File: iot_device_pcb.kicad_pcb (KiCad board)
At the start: 2 copper layers, 71 parts, among them J1 B2B-PH-K-S_LF__SN_, J2 USB_C_Receptacle_USB2.0_16P, J3 Screw_Terminal_01x03, J4 Conn_01x04_Pin, J5 Conn_01x04_Pin, J6 Conn_01x07_Pin, K1 RAYEX-L90, Q1 BC817, Q2 BC817, Q3 BC817, U1 AMS1117-3.3, U2 MCP73871, U4 ESP32-S3-WROOM-1, U5 BME280, U6 MPU-6050

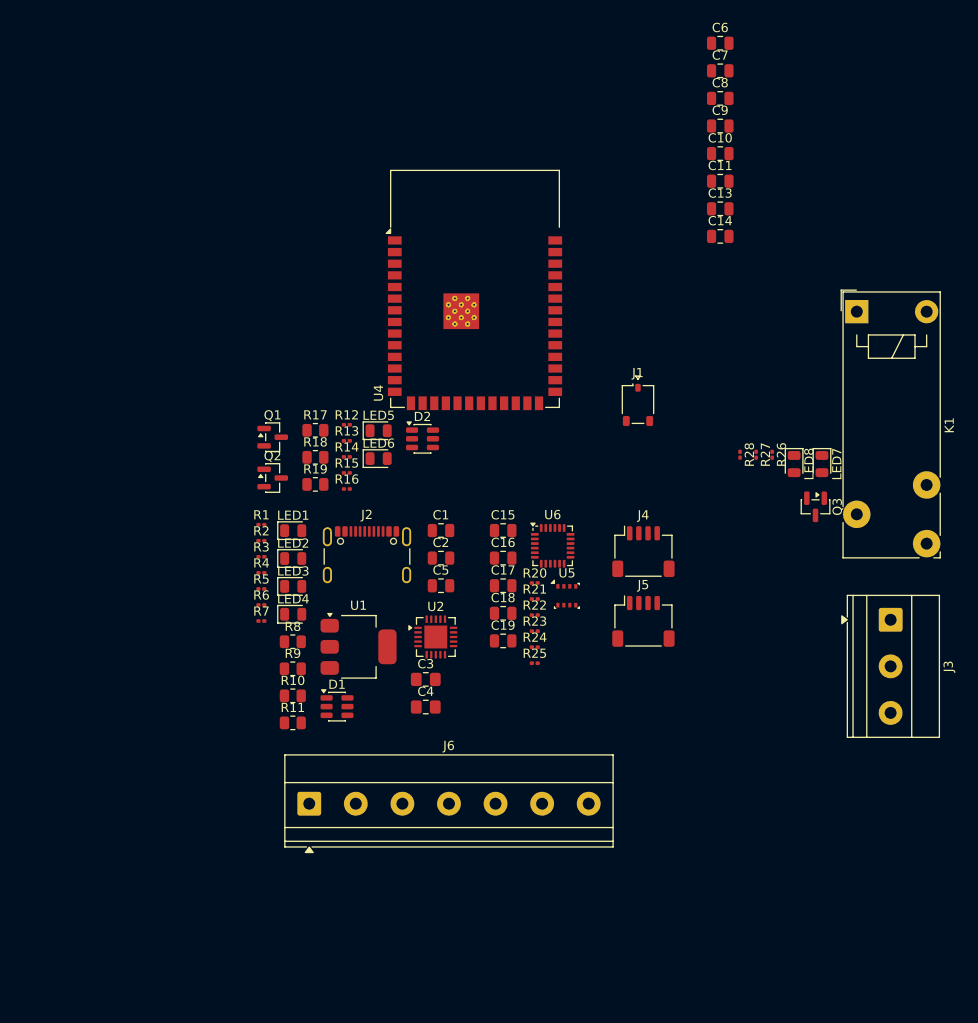
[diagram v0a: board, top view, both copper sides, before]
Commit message: Implement feature X to enhance user experience and fix bug Y in module Z
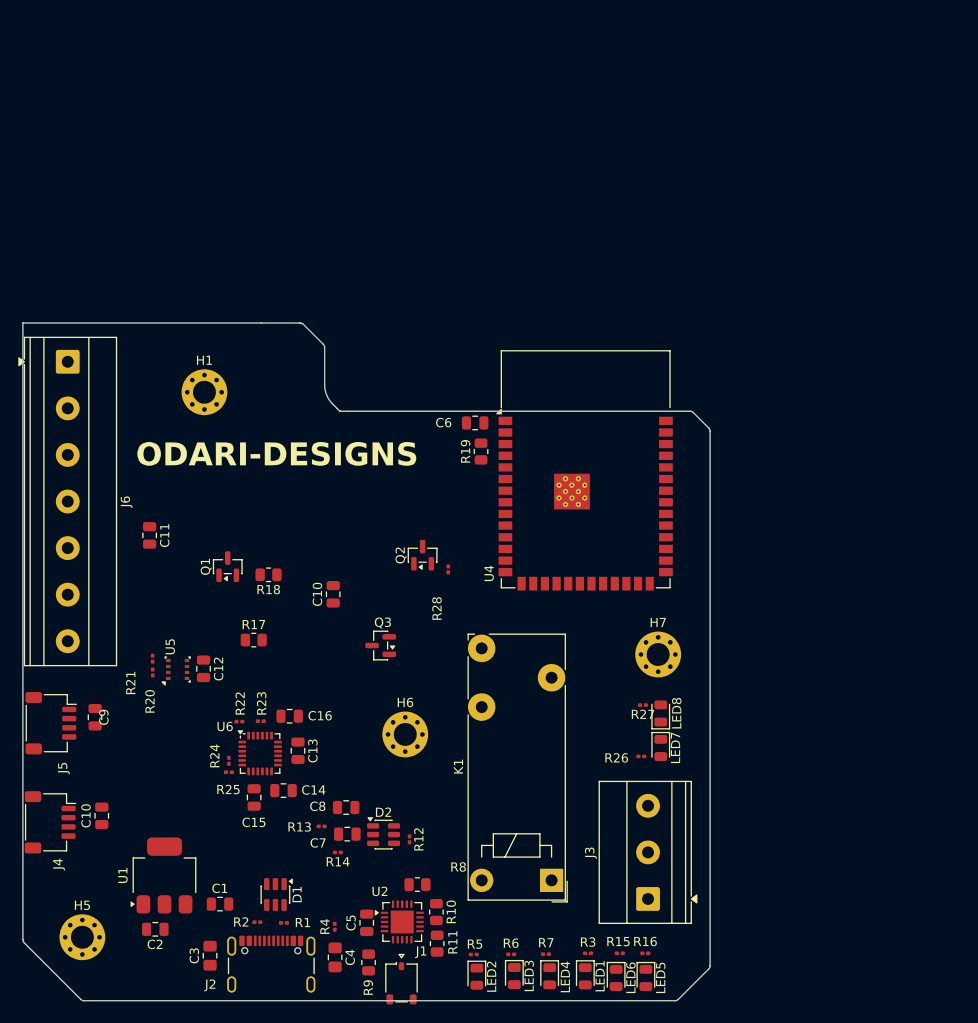
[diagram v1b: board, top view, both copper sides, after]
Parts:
- removed the C7 at (162.4, 55.2)
- added H1: MountingHole, MountingHole:MountingHole_2.5mm_Pad_Via, F.Cu at (106.1, 90.3)
- added H5: MountingHole, MountingHole:MountingHole_2.5mm_Pad_Via, F.Cu at (92.8, 149.7)
- added H6: MountingHole, MountingHole:MountingHole_2.5mm_Pad_Via, F.Cu at (128.0, 127.6)
- added H7: MountingHole, MountingHole:MountingHole_2.5mm_Pad_Via, F.Cu at (155.6, 118.9)
- moved C10 98.8 mm to (94.9, 136.5), turned to 90 degrees
- moved C9 93.9 mm to (94.2, 125.8), turned to 90 degrees
- moved C7 90.0 mm to (121.7, 138.5)
- moved C8 79.6 mm to (121.6, 135.6), turned to 180 degrees
- moved J4 71.1 mm to (89.3, 137.2), turned to -90 degrees
- moved K1 70.4 mm to (144.0, 143.5), turned to 90 degrees
- moved C11 70.3 mm to (100.1, 105.9), turned to -90 degrees
- moved J1 68.2 mm to (127.6, 154.8)
- moved LED5 66.4 mm to (154.2, 154.2), turned to -90 degrees
- moved J5 65.6 mm to (89.3, 126.4), turned to -90 degrees
- moved LED6 62.3 mm to (151.0, 154.2), turned to -90 degrees
- moved R15 60.3 mm to (151.4, 151.5), turned to 180 degrees
- moved R16 60.2 mm to (154.2, 151.5), turned to 180 degrees
- moved C10 59.6 mm to (120.1, 112.3), turned to 90 degrees
- moved LED1 58.1 mm to (147.6, 154.0), turned to -90 degrees
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- renumbered C13 to C10, C14 to C11, C15 to C12, C16 to C13, C17 to C14, C18 to C15, C19 to C16, C8 to C7, C11 to C8
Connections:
- U4 pad 12: unconnected-(U4-IO8-Pad12) -> /Microcontroller-ESP32-S3-WROOM-1/SDA
- U4 pad 15: unconnected-(U4-IO3-Pad15) -> /Microcontroller-ESP32-S3-WROOM-1/GPIO1
- U4 pad 17: unconnected-(U4-IO9-Pad17) -> /Microcontroller-ESP32-S3-WROOM-1/SCL
- U4 pad 18: unconnected-(U4-IO10-Pad18) -> /Microcontroller-ESP32-S3-WROOM-1/RELAY_FAN_GPIO
- U4 pad 19: unconnected-(U4-IO11-Pad19) -> /Microcontroller-ESP32-S3-WROOM-1/INT
- U4 pad 38: unconnected-(U4-IO2-Pad38) -> /Microcontroller-ESP32-S3-WROOM-1/GPIO1
- U4 pad 39: unconnected-(U4-IO1-Pad39) -> /Microcontroller-ESP32-S3-WROOM-1/GPIO1
- U4 pad 4: unconnected-(U4-IO4-Pad4) -> /Microcontroller-ESP32-S3-WROOM-1/GPIO1
- U4 pad 5: unconnected-(U4-IO5-Pad5) -> /Microcontroller-ESP32-S3-WROOM-1/GPIO1
- U4 pad 6: unconnected-(U4-IO6-Pad6) -> /Microcontroller-ESP32-S3-WROOM-1/GPIO1
- U4 pad 7: unconnected-(U4-IO7-Pad7) -> /Microcontroller-ESP32-S3-WROOM-1/GPIO1
- U6 pad 9: /Microcontroller-ESP32-S3-WROOM-1/ADO -> GND
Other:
- board outline added: 75 x 73.9 mm
- board text added: "ODARI-DESIGNS"
